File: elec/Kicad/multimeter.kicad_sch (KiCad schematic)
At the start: 8 parts, among them J3 HX0201800000G

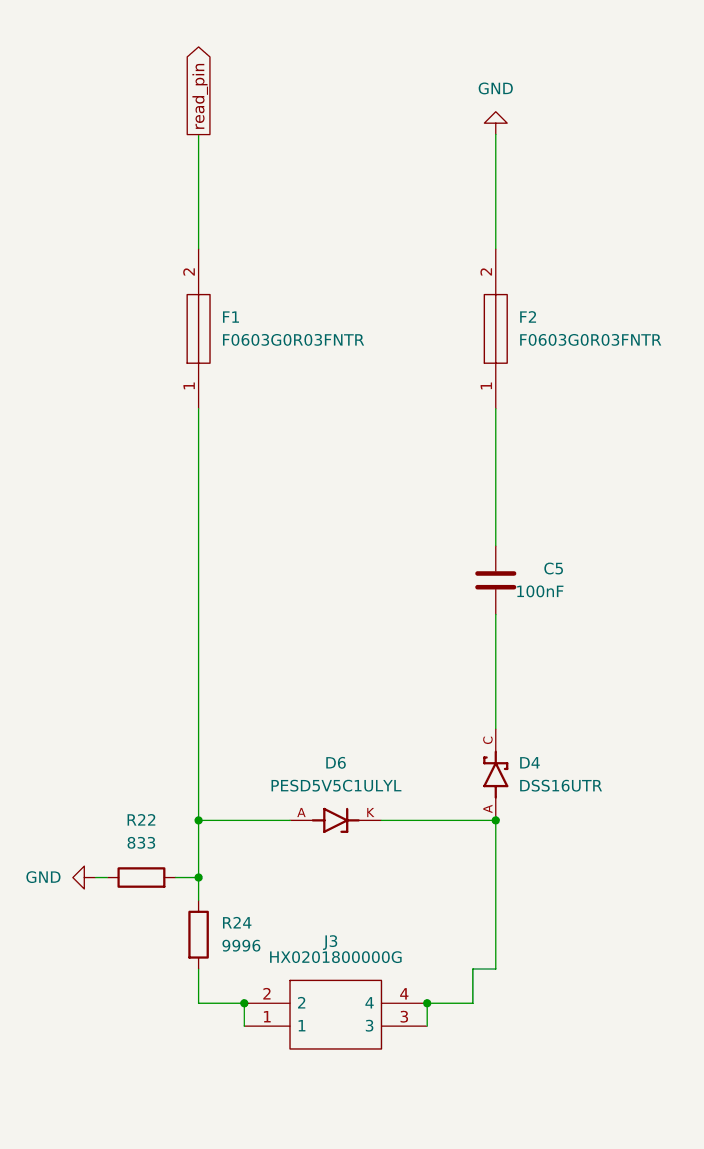
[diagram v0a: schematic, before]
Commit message: jpense qu'on est ready to order
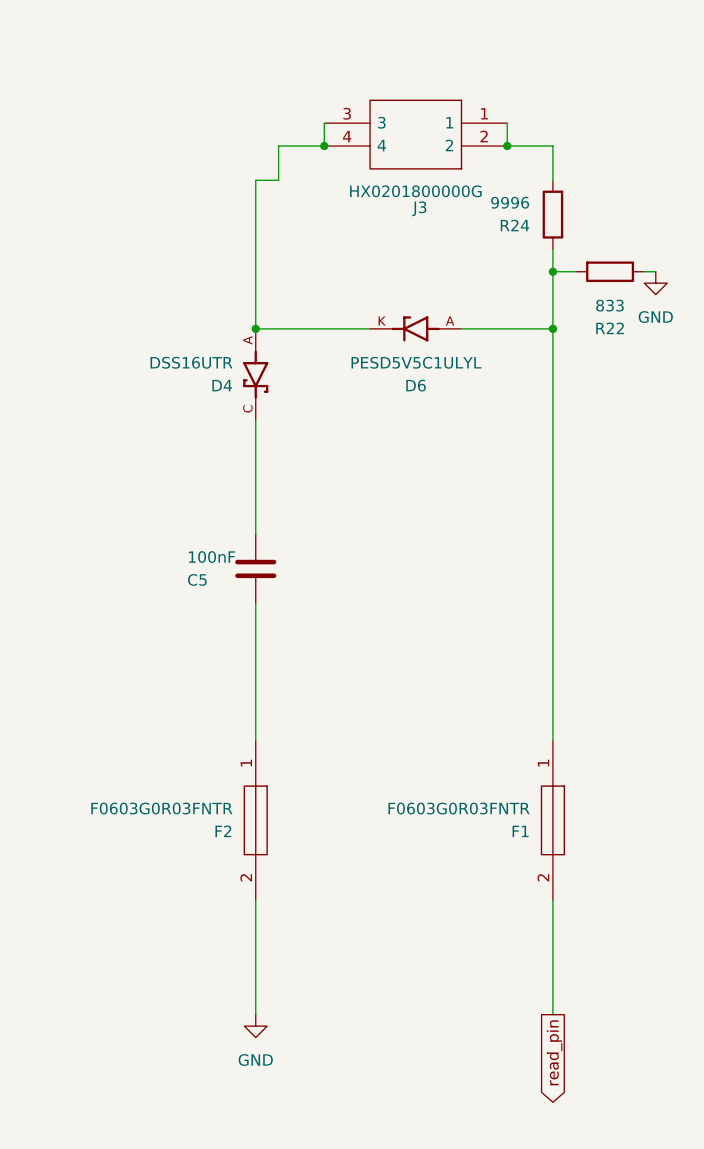
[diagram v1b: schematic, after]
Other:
- moved on the sheet: C5, D4, D6, F1, F2, J3, R22, R24
